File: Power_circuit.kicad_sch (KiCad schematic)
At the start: 13 parts, among them U1 LNK3206D

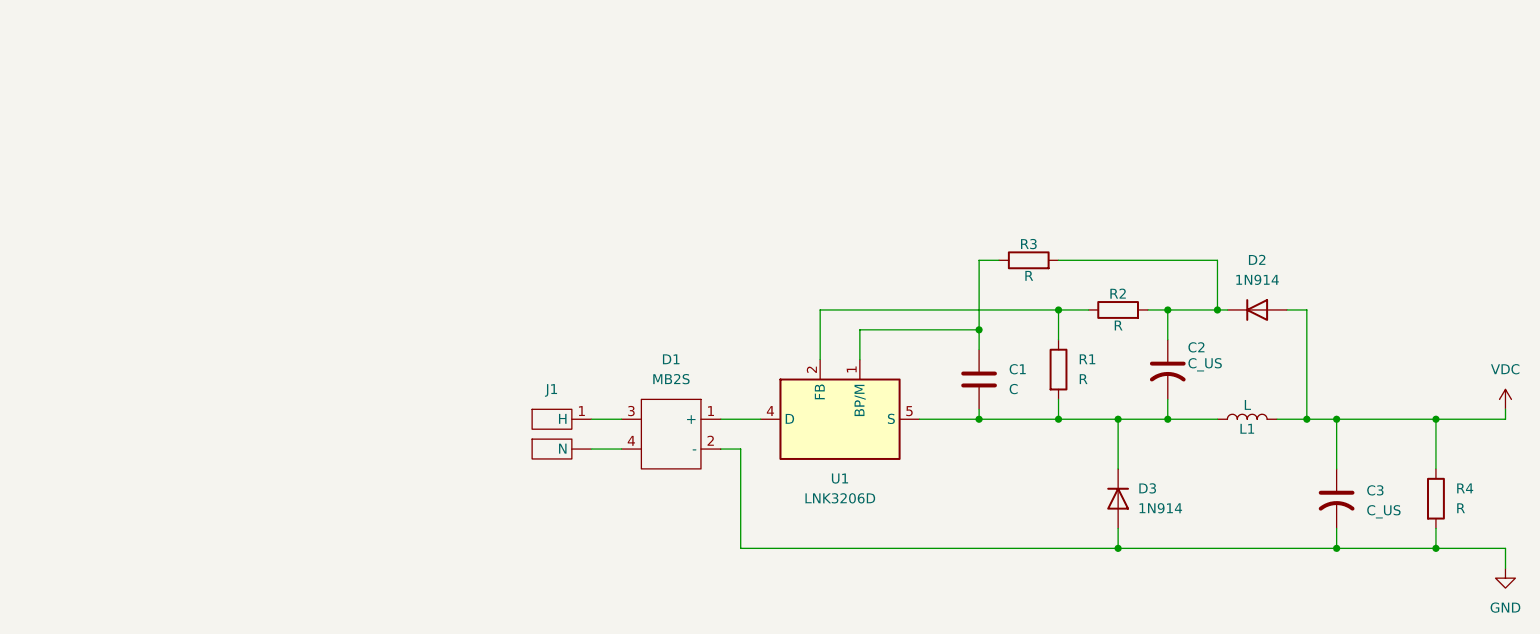
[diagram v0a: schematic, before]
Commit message: Ninth commit, power circuit
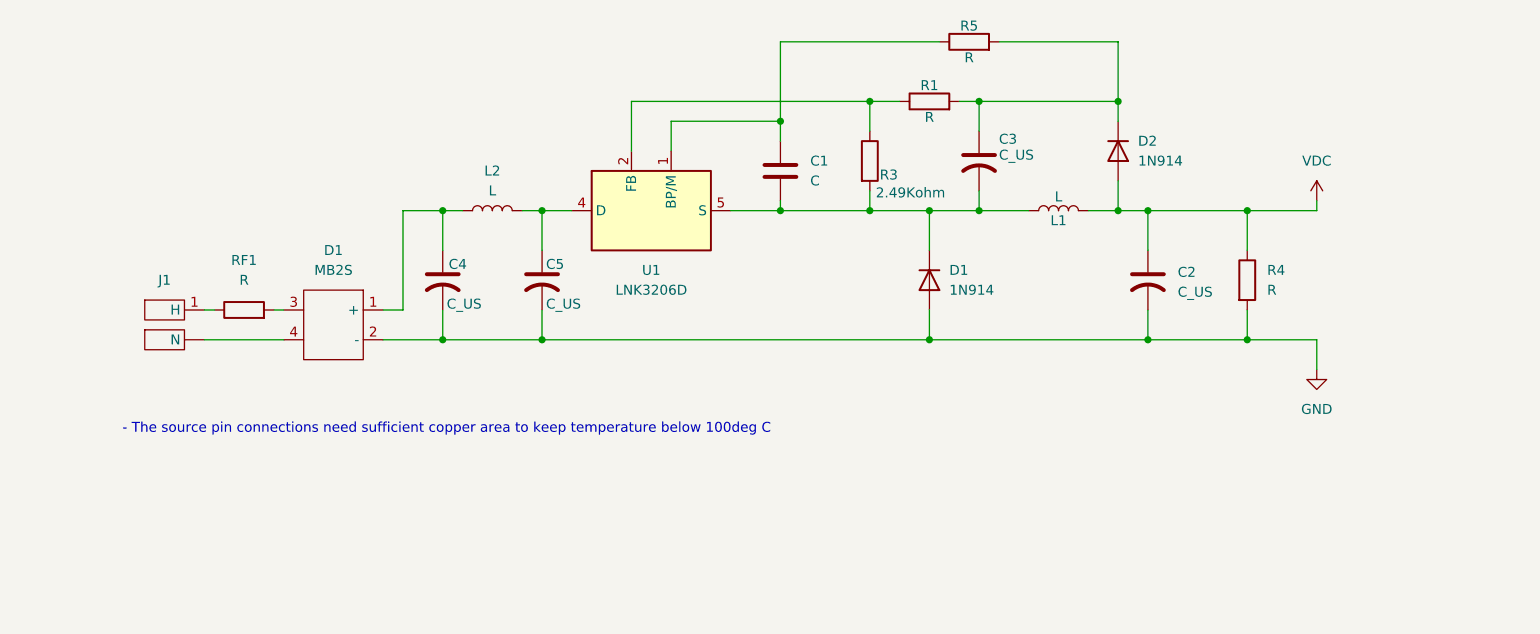
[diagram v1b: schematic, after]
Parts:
- added C4, C5: C_US, symbol Device:C_US
- added L2: L, symbol Device:L
- added RF1: R, symbol Device:R
- R3: renamed from R1; value R -> 2.49Kohm
- renumbered C3 to C2, C2 to C3, D3 to D1, R2 to R1, R3 to R5
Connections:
- net GND: now also C4.2, C5.2
- net at J1.1 (H): now also RF1.1; no longer D1.3
- net at D1.1 (+): now also C4.1, L2.1; no longer U1.4 (D)
- new net: D1.3, RF1.2
- new net: C5.1, L2.2, U1.4 (D)
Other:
- note added: "- The source pin connections need sufficient copper area to keep temperature below 100deg C"
- moved on the sheet: C1, C2, C3, D1, D2, J1, L1, R1, R3, R4, R5, U1
